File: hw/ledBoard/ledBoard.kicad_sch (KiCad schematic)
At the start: 36 parts, among them J1 Conn_01x13_Socket, J2 Conn_01x13_Socket, J6 726386-2, J7 726386-2, Q1 NMOS, Q2 NMOS, U1 INA180A1, U4 LM5148RGYR

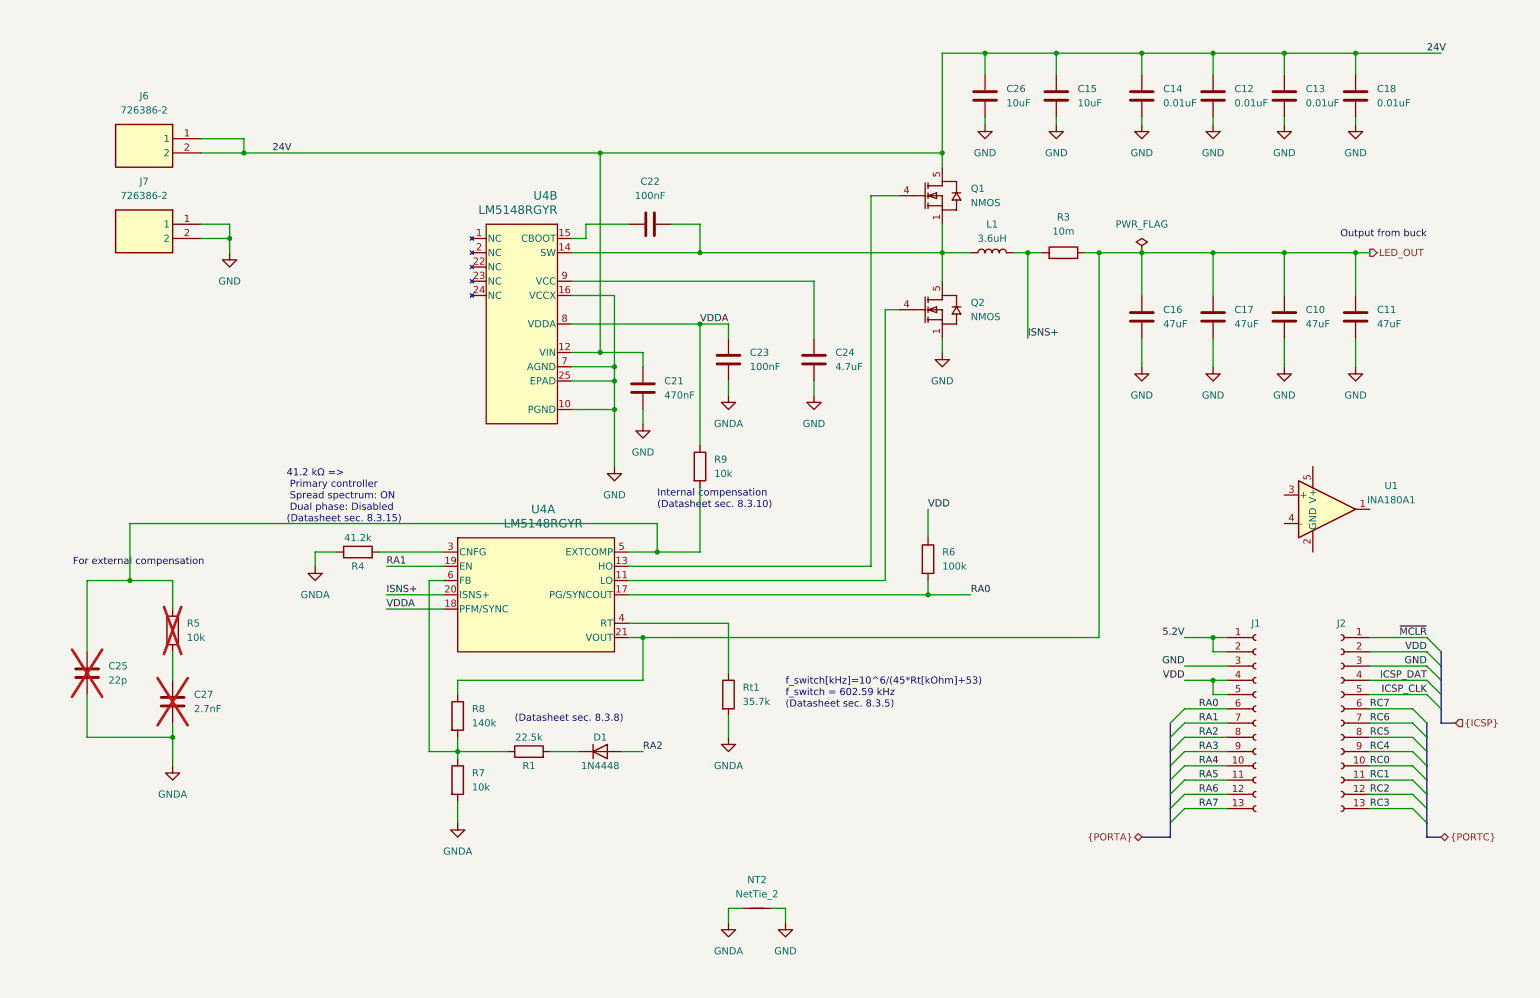
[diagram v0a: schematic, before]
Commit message: hw - ledBoard
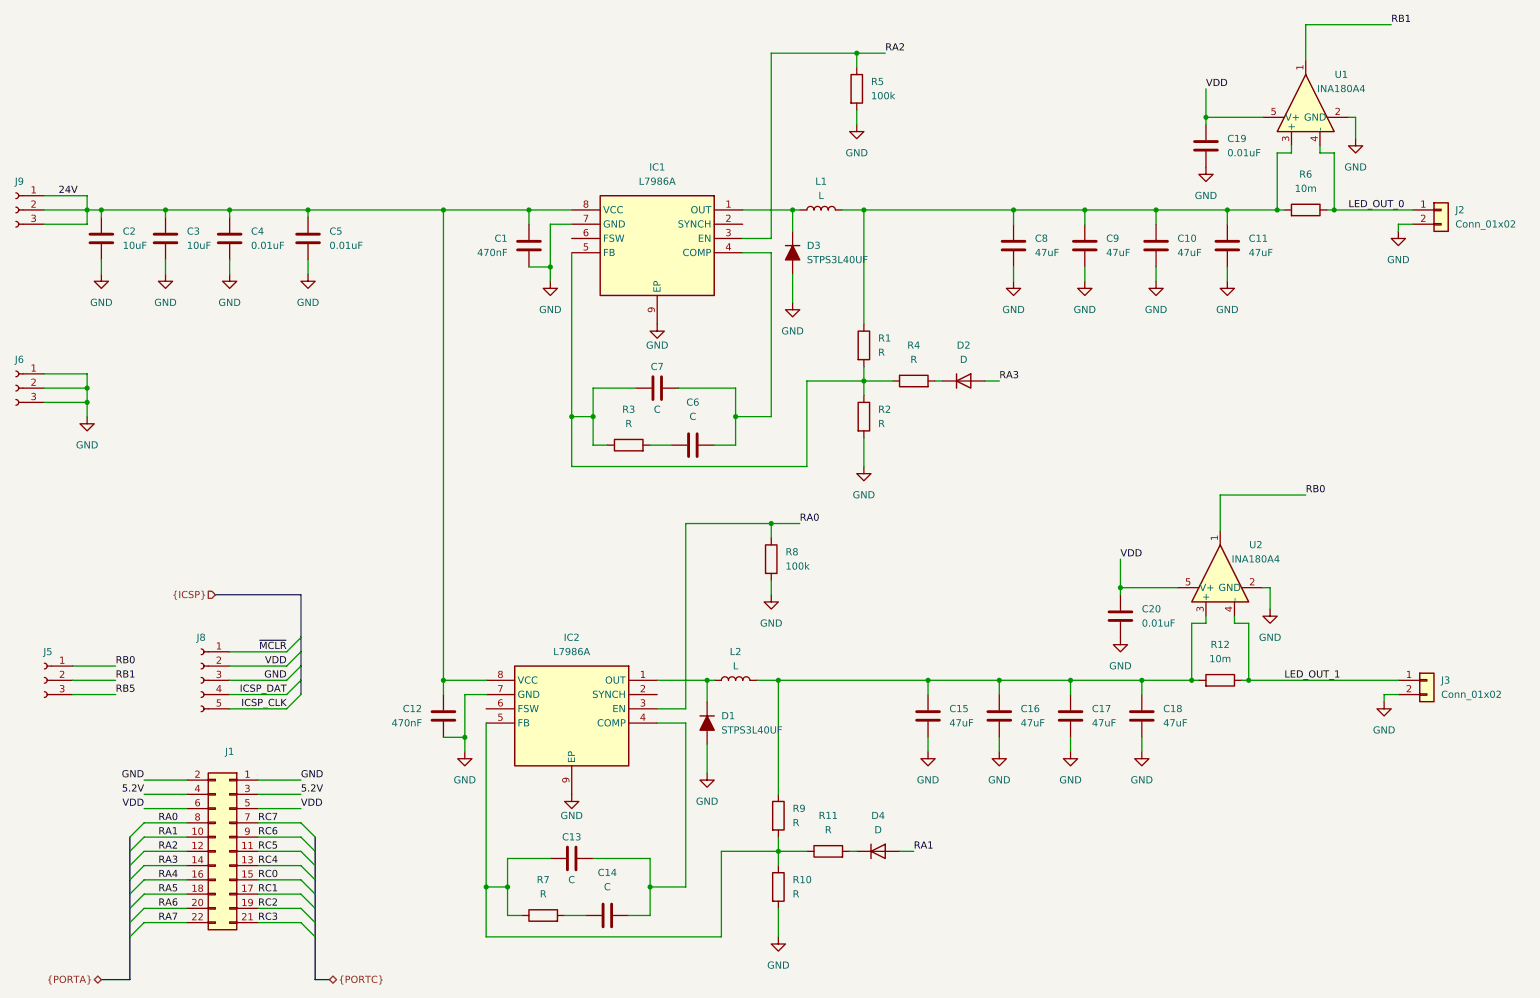
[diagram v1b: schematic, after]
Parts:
- removed C21: 470nF, Capacitor_SMD:C_0805_2012Metric_Pad1.18x1.45mm_HandSolder, symbol Device:C
- removed C22, C23: 100nF, Capacitor_SMD:C_0805_2012Metric_Pad1.18x1.45mm_HandSolder, symbol Device:C
- removed C24: 4.7uF, Capacitor_SMD:C_0805_2012Metric_Pad1.18x1.45mm_HandSolder, symbol Device:C
- removed C25: 22p, Capacitor_SMD:C_0805_2012Metric_Pad1.18x1.45mm_HandSolder, symbol Device:C
- removed C26: 10uF, Capacitor_SMD:C_1210_3225Metric_Pad1.33x2.70mm_HandSolder, symbol Device:C
- removed C27: 2.7nF, Capacitor_SMD:C_0805_2012Metric_Pad1.18x1.45mm_HandSolder, symbol Device:C
- removed D1: 1N4448, Diode_SMD:D_SOD-523, symbol Diode:1N4448
- removed J2: Conn_01x13_Socket, Connector_PinSocket_2.54mm:PinSocket_1x13_P2.54mm_Vertical, symbol Connector:Conn_01x13_Socket
- removed J6, J7: 726386-2, 726386-2, symbol FASTON:726386-2
- removed NT2: NetTie_2, NetTie:NetTie-2_SMD_Pad0.5mm, symbol Device:NetTie_2
- removed Q1, Q2: NMOS, NMOS-CSD18514:DQJ0008A, symbol NMOS-CSD18514:CSD18514Q5A
- removed Rt1: 35.7k, Resistor_SMD:R_0805_2012Metric_Pad1.20x1.40mm_HandSolder, symbol Device:R
- removed U1: INA180A1, Package_TO_SOT_SMD:SOT-23-5, symbol Amplifier_Current:INA180A1
- removed U4: LM5148RGYR, LM5148:VQFN24_RGY_TEX, symbol LM5148:LM5148RGYR
- added C1: 470nF, Capacitor_SMD:C_0805_2012Metric_Pad1.18x1.45mm_HandSolder, symbol Device:C
- added C19, C20, C4, C5: 0.01uF, Capacitor_SMD:C_0805_2012Metric_Pad1.18x1.45mm_HandSolder, symbol Device:C
- added C2, C3: 10uF, Capacitor_SMD:C_1210_3225Metric_Pad1.33x2.70mm_HandSolder, symbol Device:C
- added C6, C7: C, Capacitor_SMD:C_0805_2012Metric_Pad1.18x1.45mm_HandSolder, symbol Device:C
- added C8, C9: 47uF, Capacitor_SMD:C_1210_3225Metric_Pad1.33x2.70mm_HandSolder, symbol Device:C
- added D1, D3: STPS3L40UF, SODFL5436X110N, symbol STPS3L40:STPS3L40UF
- added D2, D4: D, Diode_SMD:D_SOD-523, symbol Device:D
- added IC1, IC2: L7986A, SOIC127P600X170-9N, symbol L7986A:L7986A
- added J2, J3: Conn_01x02, Connector_JST:JST_XH_B2B-XH-A_1x02_P2.50mm_Vertical, symbol Connector_Generic:Conn_01x02
- added J5, J6, J9: Conn_01x03_Socket, Connector_PinSocket_2.54mm:PinSocket_1x03_P2.54mm_Vertical, symbol Connector:Conn_01x03_Socket
- added J8: Conn_01x05_Socket, Connector_PinSocket_2.54mm:PinSocket_1x05_P2.54mm_Vertical, symbol Connector:Conn_01x05_Socket
- added L2: L, Inductor_SMD:L_Bourns-SRN8040_8x8.15mm, symbol Device:L
- added R10, R11, R2: R, Resistor_SMD:R_0805_2012Metric_Pad1.20x1.40mm_HandSolder, symbol Device:R
- added R12: 10m, Resistor_SMD:R_0815_2038Metric_Pad1.20x4.05mm_HandSolder, symbol Device:R
- added U1, U2: INA180A4, Package_TO_SOT_SMD:SOT-23-5, symbol Amplifier_Current:INA180A4
- C12: value 0.01uF -> 470nF
- C13, C14: value 0.01uF -> C
- C15: value 10uF -> 47uF
- C18: value 0.01uF -> 47uF; footprint Capacitor_SMD:C_0805_2012Metric_Pad1.18x1.45mm_HandSolder -> Capacitor_SMD:C_1210_3225Metric_Pad1.33x2.70mm_HandSolder
- J1: value Conn_01x13_Socket -> Conn_02x11_Socket; footprint Connector_PinSocket_2.54mm:PinSocket_1x13_P2.54mm_Vertical -> Library:LedBoardPinHeader; symbol Connector:Conn_01x13_Socket -> Connector_Generic:Conn_02x11_Odd_Even
- L1: value 3.6uH -> L
- R1: value 22.5k -> R
- R3: value 10m -> R; footprint Resistor_SMD:R_0815_2038Metric_Pad1.20x4.05mm_HandSolder -> Resistor_SMD:R_0805_2012Metric_Pad1.20x1.40mm_HandSolder
- R4: value 41.2k -> R
- R5: value 10k -> 100k; now fitted
- R6: value 100k -> 10m; footprint Resistor_SMD:R_0805_2012Metric_Pad1.20x1.40mm_HandSolder -> Resistor_SMD:R_0815_2038Metric_Pad1.20x4.05mm_HandSolder
- R7, R9: value 10k -> R
- R8: value 140k -> 100k
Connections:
- net 24V: now also C1.1, C2.1, C3.1, C4.1, C5.1, IC1.8 (VCC), IC2.8 (VCC), J9.1 (Pin_1), J9.2 (Pin_2), J9.3 (Pin_3); no longer C13.1, C14.1, C15.1, C18.1
- net 5.2V: now also J1.3 (Pin_3), J1.4 (Pin_4); no longer J1.1 (Pin_1), J1.2 (Pin_2)
- net GND: now also J1.1 (Pin_1), J1.2 (Pin_2), R5.2, R8.2, C1.2, C19.2, C2.2, C20.2, C3.2, C4.2, C5.2, C8.2, C9.2, D1.2 (A), D3.2 (A), IC1.7 (GND), IC1.9 (EP), IC2.7 (GND), IC2.9 (EP), J2.2 (Pin_2), J3.2 (Pin_2), J6.1 (Pin_1), J6.2 (Pin_2), J6.3 (Pin_3), J8.3 (Pin_3), R10.2, R2.2, U1.2 (GND), U2.2 (GND); no longer C13.2, C14.2, J1.3 (Pin_3)
- net ICSP_CLK: now also J8.5 (Pin_5)
- net ICSP_DAT: now also J8.4 (Pin_4)
- net RA0: now also J1.8 (Pin_8), R8.1, IC2.3 (EN); no longer J1.6 (Pin_6), R6.2
- net RA1: now also J1.10 (Pin_10), D4.2 (A); no longer J1.7 (Pin_7)
- net RA2: now also J1.12 (Pin_12), R5.1, IC1.3 (EN); no longer J1.8 (Pin_8)
- net RA3: now also J1.14 (Pin_14), D2.2 (A); no longer J1.9 (Pin_9)
- net RA4: now also J1.16 (Pin_16); no longer J1.10 (Pin_10)
- net RA5: now also J1.18 (Pin_18); no longer J1.11 (Pin_11)
- net RA6: now also J1.20 (Pin_20); no longer J1.12 (Pin_12)
- net RA7: now also J1.22 (Pin_22); no longer J1.13 (Pin_13)
- net RC0: now also J1.15 (Pin_15)
- net RC1: now also J1.17 (Pin_17)
- net RC2: now also J1.19 (Pin_19)
- net RC3: now also J1.21 (Pin_21)
- net RC4: now also J1.13 (Pin_13)
- net RC5: now also J1.11 (Pin_11)
- net RC6: now also J1.9 (Pin_9)
- net RC7: now also J1.7 (Pin_7)
- net VDD: now also J1.6 (Pin_6), C19.1, C20.1, J8.2 (Pin_2), U1.5 (V+), U2.5 (V+); no longer J1.4 (Pin_4), R6.1
- net ~{MCLR}: now also J8.1 (Pin_1)
- net at R1.2: now also R3.1, R4.1, C7.2, IC1.5 (FB), R2.1
- net at R9.2: now also C13.2, R7.1, IC2.5 (FB), R10.1, R11.1; no longer R5.1
- net at L1.2: now also D3.1 (K), IC1.1 (OUT)
- net at R4.2: now also D2.1 (K)
- net GNDA: no longer names the net of R7.2
- net GNDA: now also C14.2; no longer R4.1
- net ISNS+: no longer names the net of R3.2
- net ISNS+: now also C6.2; no longer L1.1
- removed net LED_OUT: C10.1, C11.1, C16.1, C17.1, R3.1, R8.1
- net VDDA: no longer names the net of R9.1
- net VDDA: now also C15.1, C16.1, C17.1, C18.1, L2.1, R12.2, U2.3 (+)
- new net: C13.1, C14.1, IC2.4 (COMP)
- new net: C6.1, C7.1, IC1.4 (COMP)
- new net: C10.1, C11.1, C8.1, C9.1, L1.1, R1.1, R6.2, U1.3 (+)
- new net: D4.1 (K), R11.2
- new net: D1.1 (K), IC2.1 (OUT), L2.2
- new net LED_OUT_0: J2.1 (Pin_1), R6.1, U1.4 (-)
- new net LED_OUT_1: J3.1 (Pin_1), R12.1, U2.4 (-)
- new net RB0: J5.1 (Pin_1), U2.1
- new net RB1: J5.2 (Pin_2), U1.1
- new net RB5: J5.3 (Pin_3)
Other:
- note removed: "(Datasheet sec. 8.3.8)"
- note removed: "41.2 kΩ => Primary controller Spread spectrum: ON Dual phase: Disabled (Datasheet sec. 8.3.15)"
- note removed: "For external compensation"
- note removed: "Internal compensation (Datasheet sec. 8.3.10)"
- note removed: "Output from buck"
- note removed: "f_switch[kHz]=10^6/(45*Rt[kOhm]+53) f_switch = 602.59 kHz (Datasheet sec. 8.3.5)"
